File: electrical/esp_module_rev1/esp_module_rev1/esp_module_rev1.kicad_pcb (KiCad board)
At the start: 4 copper layers, 47.2 x 47 mm, 66 parts, among them J1 USB_C_Receptacle_USB2.0_14P, J3 Conn_01x02, Q1 FDN340P, Q2 FDN340P, SW1 SW_Push, SW2 SW_Push, U1 MCP73831-2-OT, U10 BMP390L, U2 USBLC6-2SC6, U3 TLV75533PDBV, U4 TLV75518PDBV, U5 ESP32-C3-WROOM-02, U6 TXS0102DCT, U7 INA180A1, U8 LSM6DS3, U9 MAX30102

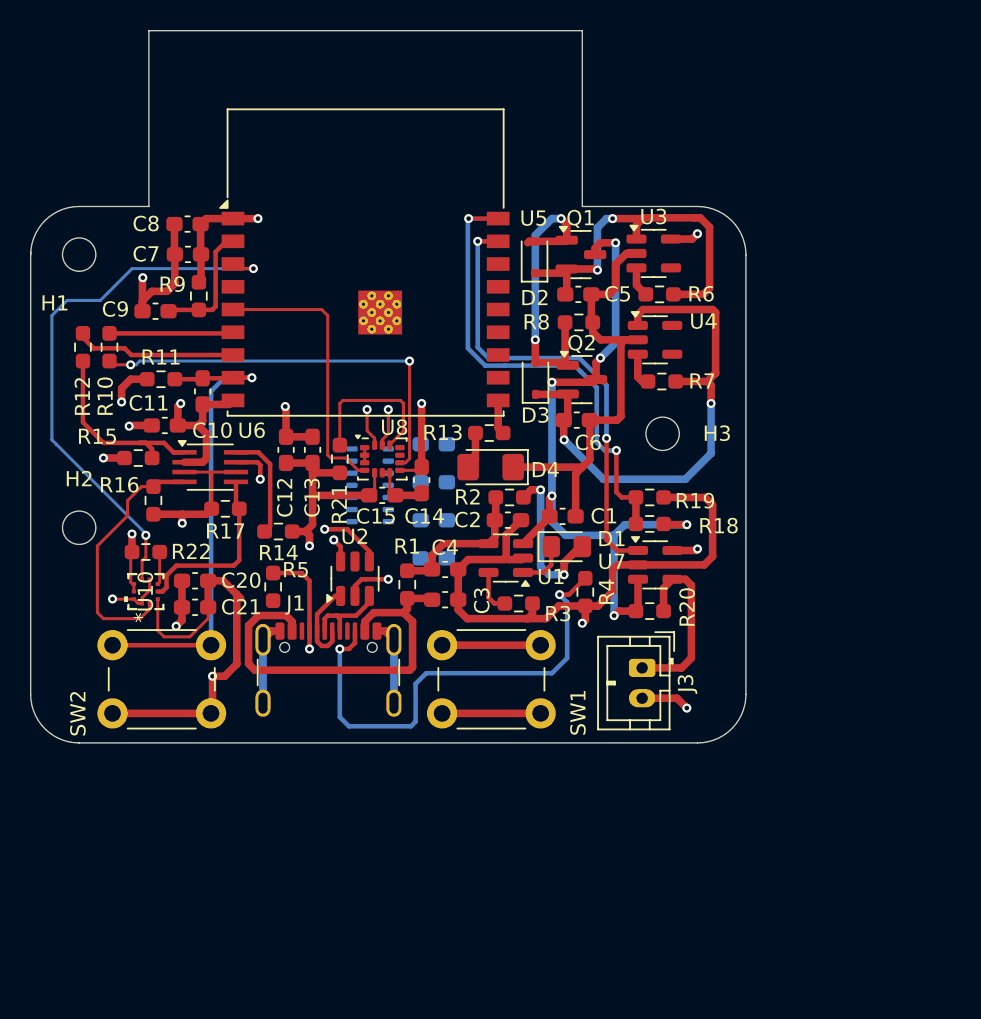
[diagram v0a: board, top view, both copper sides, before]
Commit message: Layout attempt two. Routing started
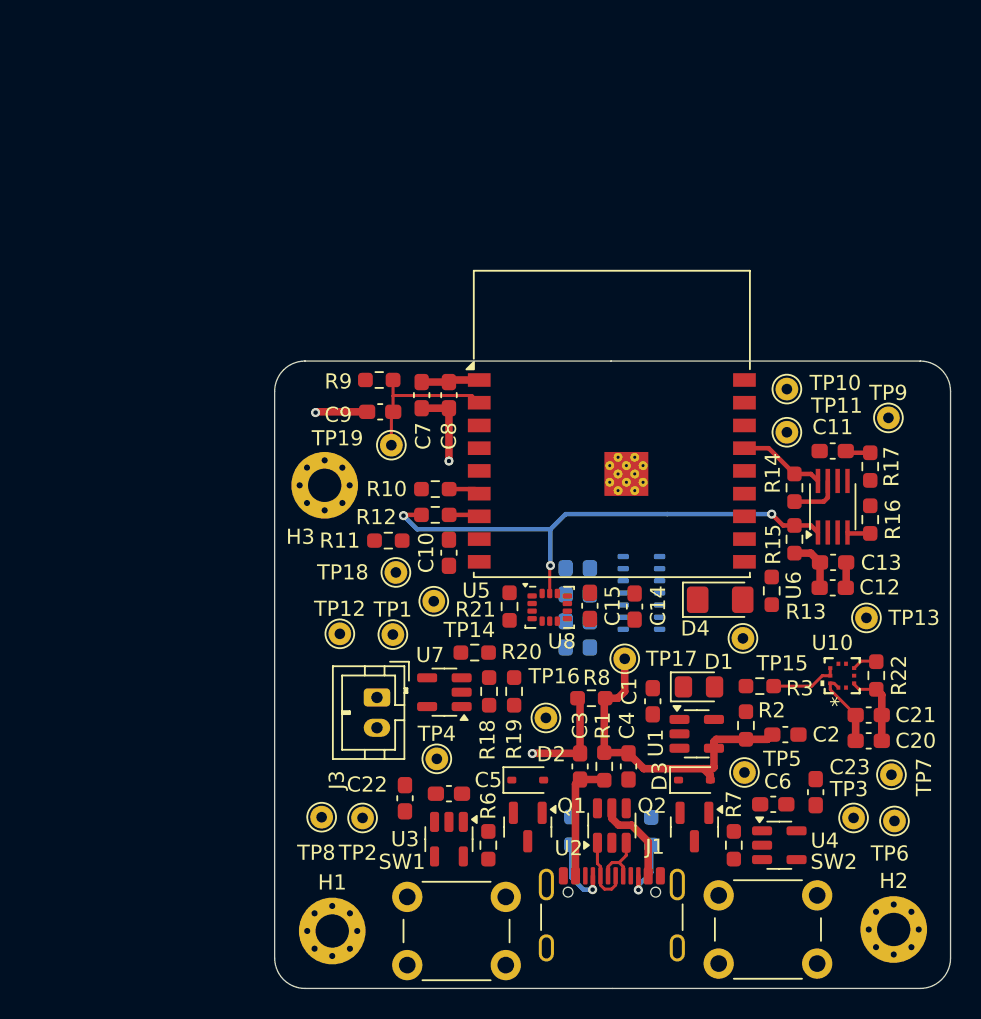
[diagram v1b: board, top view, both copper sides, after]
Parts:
- added C22: 1uF, Capacitor_SMD:C_0603_1608Metric_Pad1.08x0.95mm_HandSolder, F.Cu at (134.1, 110.8)
- added C23: 1uF, Capacitor_SMD:C_0603_1608Metric_Pad1.08x0.95mm_HandSolder, F.Cu at (161.2, 110.5)
- added TP1: TestPoint, TestPoint:TestPoint_THTPad_D1.5mm_Drill0.7mm, F.Cu at (133.3, 100.0)
- added TP10: TestPoint, TestPoint:TestPoint_THTPad_D1.5mm_Drill0.7mm, F.Cu at (159.3, 83.8)
- added TP11: TestPoint, TestPoint:TestPoint_THTPad_D1.5mm_Drill0.7mm, F.Cu at (159.3, 86.7)
- added TP12: TestPoint, TestPoint:TestPoint_THTPad_D1.5mm_Drill0.7mm, F.Cu at (129.8, 100.0)
- added TP13: TestPoint, TestPoint:TestPoint_THTPad_D1.5mm_Drill0.7mm, F.Cu at (164.6, 99.0)
- added TP14: TestPoint, TestPoint:TestPoint_THTPad_D1.5mm_Drill0.7mm, F.Cu at (136.0, 97.8)
- added TP15: TestPoint, TestPoint:TestPoint_THTPad_D1.5mm_Drill0.7mm, F.Cu at (156.4, 100.3)
- added TP16: TestPoint, TestPoint:TestPoint_THTPad_D1.5mm_Drill0.7mm, F.Cu at (143.4, 105.5)
- added TP17: TestPoint, TestPoint:TestPoint_THTPad_D1.5mm_Drill0.7mm, F.Cu at (148.6, 101.7)
- added TP18: TestPoint, TestPoint:TestPoint_THTPad_D1.5mm_Drill0.7mm, F.Cu at (133.5, 96.0)
- added TP19: TestPoint, TestPoint:TestPoint_THTPad_D1.5mm_Drill0.7mm, F.Cu at (133.2, 87.5)
- added TP2: TestPoint, TestPoint:TestPoint_THTPad_D1.5mm_Drill0.7mm, F.Cu at (131.3, 112.2)
- added TP3: TestPoint, TestPoint:TestPoint_THTPad_D1.5mm_Drill0.7mm, F.Cu at (163.7, 112.2)
- added TP4: TestPoint, TestPoint:TestPoint_THTPad_D1.5mm_Drill0.7mm, F.Cu at (136.2, 108.2)
- added TP5: TestPoint, TestPoint:TestPoint_THTPad_D1.5mm_Drill0.7mm, F.Cu at (156.5, 109.2)
- added TP6: TestPoint, TestPoint:TestPoint_THTPad_D1.5mm_Drill0.7mm, F.Cu at (166.4, 112.3)
- added TP7: TestPoint, TestPoint:TestPoint_THTPad_D1.5mm_Drill0.7mm, F.Cu at (166.2, 109.3)
- added TP8: TestPoint, TestPoint:TestPoint_THTPad_D1.5mm_Drill0.7mm, F.Cu at (128.6, 112.1)
- added TP9: TestPoint, TestPoint:TestPoint_THTPad_D1.5mm_Drill0.7mm, F.Cu at (166.0, 85.8)
- H1, H2, H3: value MountingHole -> MountingHole_Pad; footprint MountingHole:MountingHole_2.2mm_M2 -> MountingHole:MountingHole_2.2mm_M2_Pad_Via
- R4, R5: moved to B.Cu
- moved H2 59.9 mm to (166.3, 119.5)
- moved R22 48.9 mm to (165.2, 102.8), turned to 90 degrees
- moved H1 47.7 mm to (129.3, 119.6)
- moved R16 47.3 mm to (164.8, 92.5), turned to -90 degrees
- moved U10 46.3 mm to (162.9, 102.8)
- moved C20 45.7 mm to (164.7, 107.1)
- moved C21 45.0 mm to (164.7, 105.4)
- moved C11 44.1 mm to (162.3, 87.9), turned to 180 degrees
- moved R15 43.6 mm to (159.8, 93.8), turned to 90 degrees
- moved R17 42.6 mm to (164.8, 89.0), turned to -90 degrees
- moved U6 41.2 mm to (162.3, 91.6), turned to 90 degrees
- moved U3 40.9 mm to (137.0, 113.5), turned to -90 degrees
- moved R6 38.1 mm to (139.6, 114.0), turned to 90 degrees
- moved Q1 37.9 mm to (142.2, 112.8), turned to -90 degrees
- moved C12 37.2 mm to (162.3, 97.0), turned to 0 degrees
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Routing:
- net GND: track 151.6 -> 27.0 mm, vias 8 -> 3
- net +BATT: track 47.7 -> 0.00 mm, vias 6 -> 0
- net /BMP_INT: track 36.2 -> 0.00 mm, vias 2 -> 0
- net Net-(D3-K): track 34.6 -> 0.00 mm, vias 2 -> 0
- net /BOOT_SEL_GPIO9: track 31.5 -> 0.00 mm, vias 1 -> 0
- net /VBATT_SENSE: track 31.2 -> 0.00 mm, vias 2 -> 0
- net /CURR_SENSE: track 30.5 -> 0.00 mm, vias 2 -> 0
- net +3V3: track 39.6 -> 10.9 mm, vias 8 -> 0
- net /USB_CC2: track 31.6 -> 4.24 mm, vias 2 -> 1
- net /LSM_INT2: track 27.2 -> 0.00 mm, vias 2 -> 0
- net Net-(D2-K): track 24.9 -> 0.00 mm, vias 2 -> 0
- net /LSM_INT1: track 18.5 -> 0.00 mm
- net /I2C_SCL: track 15.7 -> 34.1 mm, vias 1 -> 3
- net /I2C_SCL_1V8: track 16.7 -> 1.53 mm
- net +USB_VBUS: track 27.5 -> 14.1 mm
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- removed copper zone on In2.Cu, net +1V8
- removed copper zone on In2.Cu, net +3V3
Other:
- board size 47.2 x 47 mm -> 44.6 x 41.4 mm
